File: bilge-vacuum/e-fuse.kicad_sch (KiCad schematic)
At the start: 21 parts, among them Q6 PSMN014-80YL, U2 TPS24751RUVR

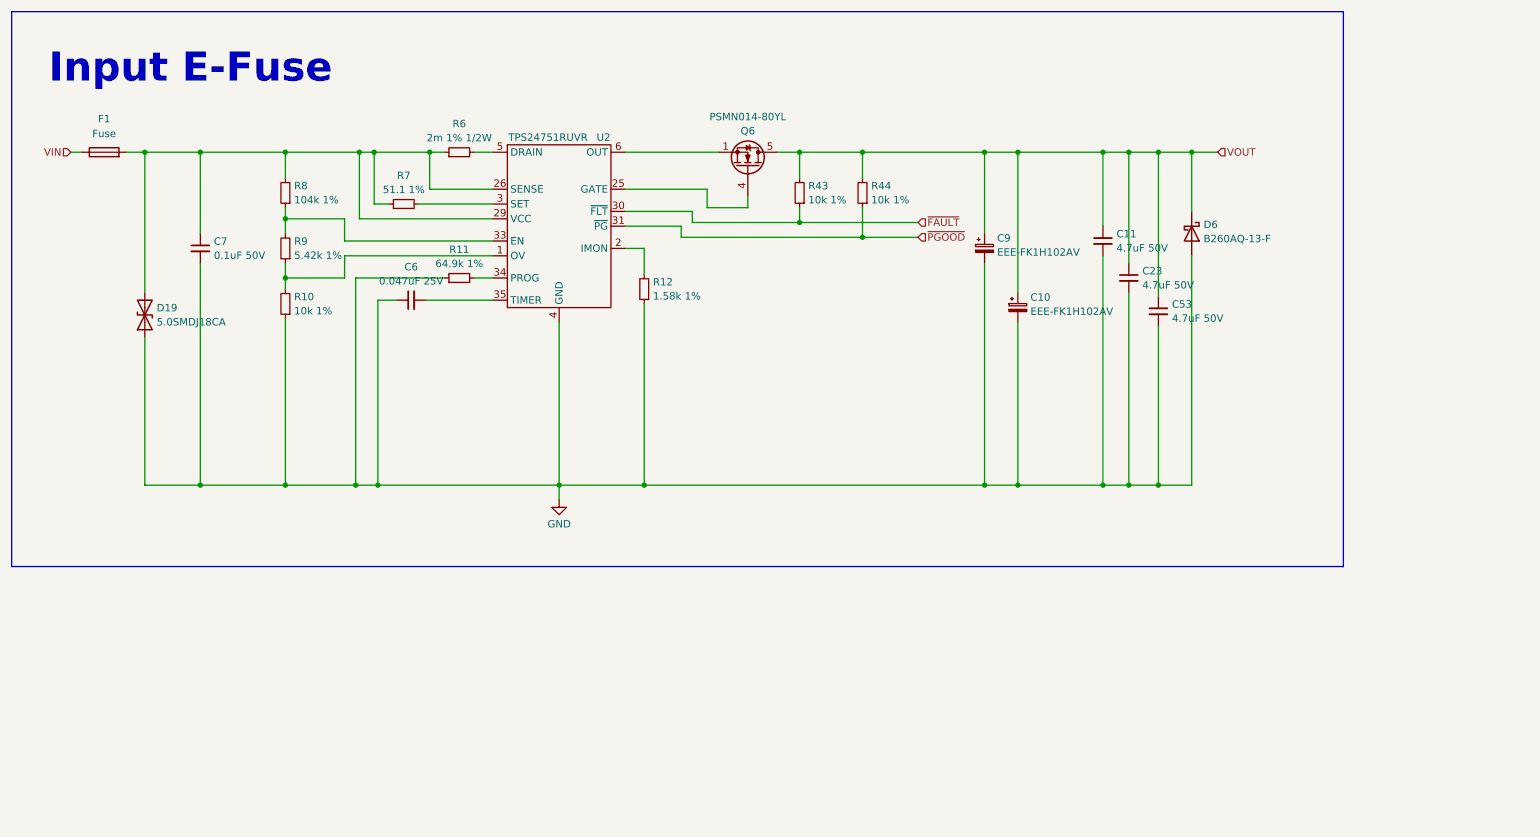
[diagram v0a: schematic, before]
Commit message: Updates
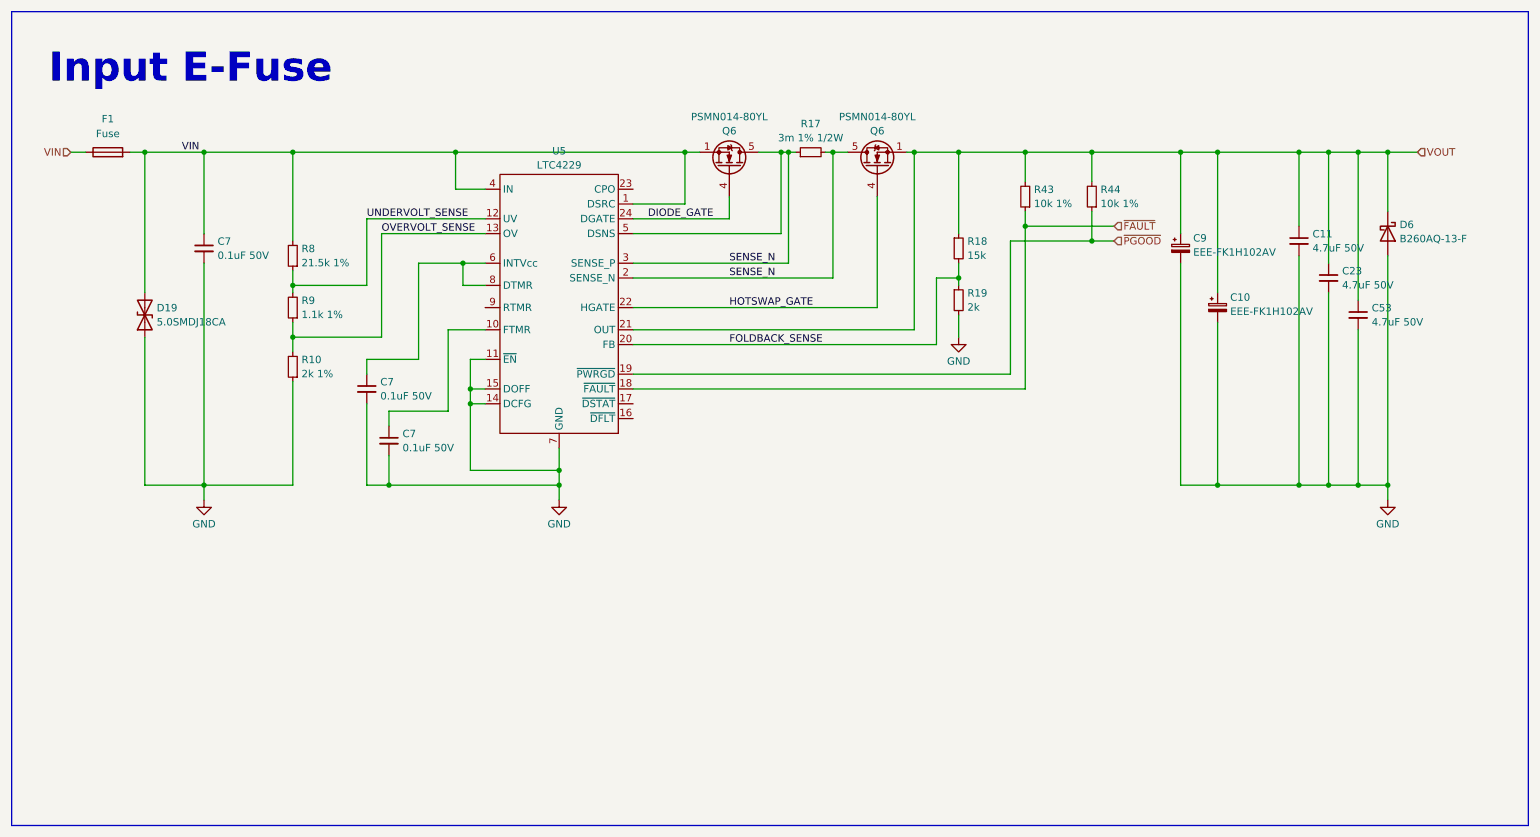
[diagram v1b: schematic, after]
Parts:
- removed C6: 0.047uF 25V, Capacitor_SMD:C_0805_2012Metric, symbol Device:C_Small
- removed R11: 64.9k 1%, Resistor_SMD:R_0805_2012Metric, symbol Device:R_Small
- removed R12: 1.58k 1%, Resistor_SMD:R_0805_2012Metric, symbol Device:R_Small
- removed R6: 2m 1% 1/2W, Resistor_SMD:R_1206_3216Metric, symbol Device:R_Small
- removed R7: 51.1 1%, Resistor_SMD:R_0805_2012Metric, symbol Device:R_Small
- removed U2: TPS24751RUVR, Custom Parts:VQFN-36, symbol Custom Parts:TPS24751RUVR
- added C7 (x2): 0.1uF 50V, Capacitor_SMD:C_0805_2012Metric, symbol Device:C_Small
- added Q6: PSMN014-80YL, Package_TO_SOT_SMD:LFPAK56, symbol Custom Parts:PSMN014-80YL
- added R17: 3m 1% 1/2W, Resistor_SMD:R_1206_3216Metric, symbol Device:R_Small
- added R18: 15k, Resistor_SMD:R_0805_2012Metric, symbol Device:R_Small
- added R19: 2k, Resistor_SMD:R_0805_2012Metric, symbol Device:R_Small
- added U5: LTC4229, Custom Parts:WFQFN-24, symbol Custom Parts:LTC4229
- R10: value 10k 1% -> 2k 1%
- R8: value 104k 1% -> 21.5k 1%
- R9: value 5.42k 1% -> 1.1k 1%
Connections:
- net GND: now also C7.2, C7.2, R19.2, U5.11 (~{EN}), U5.14 (DCFG), U5.15 (DOFF), U5.25 (GND), U5.7 (GND)
- net VIN: now also C7.1, D19.2 (A2), F1.2, R8.2, Q6.1 (S), Q6.2 (S), Q6.3 (S), U5.1 (DSRC), U5.4 (IN)
- net VOUT: now also Q6.1 (S), Q6.2 (S), Q6.3 (S), R18.1, U5.21 (OUT); no longer Q6.5 (D)
- net ~{FAULT}: now also U5.18 (~{FAULT})
- net ~{PGOOD}: now also U5.19 (~{PWRGD})
- net OVERVOLT_SENSE: now reaches R10.2, R9.1
- net OVERVOLT_SENSE: now also U5.13 (OV)
- net HOTSWAP_GATE: now reaches Q6.4 (G)
- net HOTSWAP_GATE: now also U5.22 (HGATE)
- net UNDERVOLT_SENSE: now reaches R8.1, R9.2
- net UNDERVOLT_SENSE: now also U5.12 (UV)
- new net: C7.1, U5.6 (INTVcc), U5.8 (DTMR)
- new net: C7.1, U5.10 (FTMR)
- new net DIODE_GATE: Q6.4 (G), U5.24 (DGATE)
- new net FOLDBACK_SENSE: R18.2, R19.1, U5.20 (FB)
- new net SENSE_N: Q6.5 (D), Q6.5 (D), R17.1, R17.2, U5.2 (SENSE_N), U5.3 (SENSE_P), U5.5 (DSNS)
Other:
- moved on the sheet: C10, C11, C23, C53, C7, C9, D6, F1, Q6, R10, R43, R44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
